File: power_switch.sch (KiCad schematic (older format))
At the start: 111 parts, among them IC1 ATTINY2313A-P, P1 CONN_2, P10 CONN_01X01, P11 CONN_02X01, P12 CONN_01X01, P13 CONN_2, P14 CONN_2, P15 CONN_2, P16 CONN_2, P17 CONN_2, P18 CONN_2, P19 CONN_2, P2 CONN_2, P20 CONN_2, P21 CONN_01X03, P3 CONN_2, P4 CONN_2, P5 CONN_2, P6 CONN_01X03, P7 CONN_01X01, P8 CONN_01X01, P9 CONN_01X01, Q1 Q_NPN_EBC, Q10 Q_NJFET_DGS, Q11 Q_NPN_EBC, Q12 Q_NPN_EBC, Q13 Q_NJFET_DGS, Q14 Q_NJFET_DGS, Q2 Q_NJFET_DGS, Q3 Q_NPN_EBC, Q4 Q_NPN_EBC, Q5 Q_NJFET_DGS, Q6 Q_NJFET_DGS, Q7 Q_NPN_EBC, Q8 Q_NPN_EBC, Q9 Q_NJFET_DGS, U1 LTV-817, U2 LTV-817, U3 LTV-817, U4 LTV-817, U5 LTV-817, U6 LM317T, U7 LTV-817, U8 LTV-817, U9 LTV-817

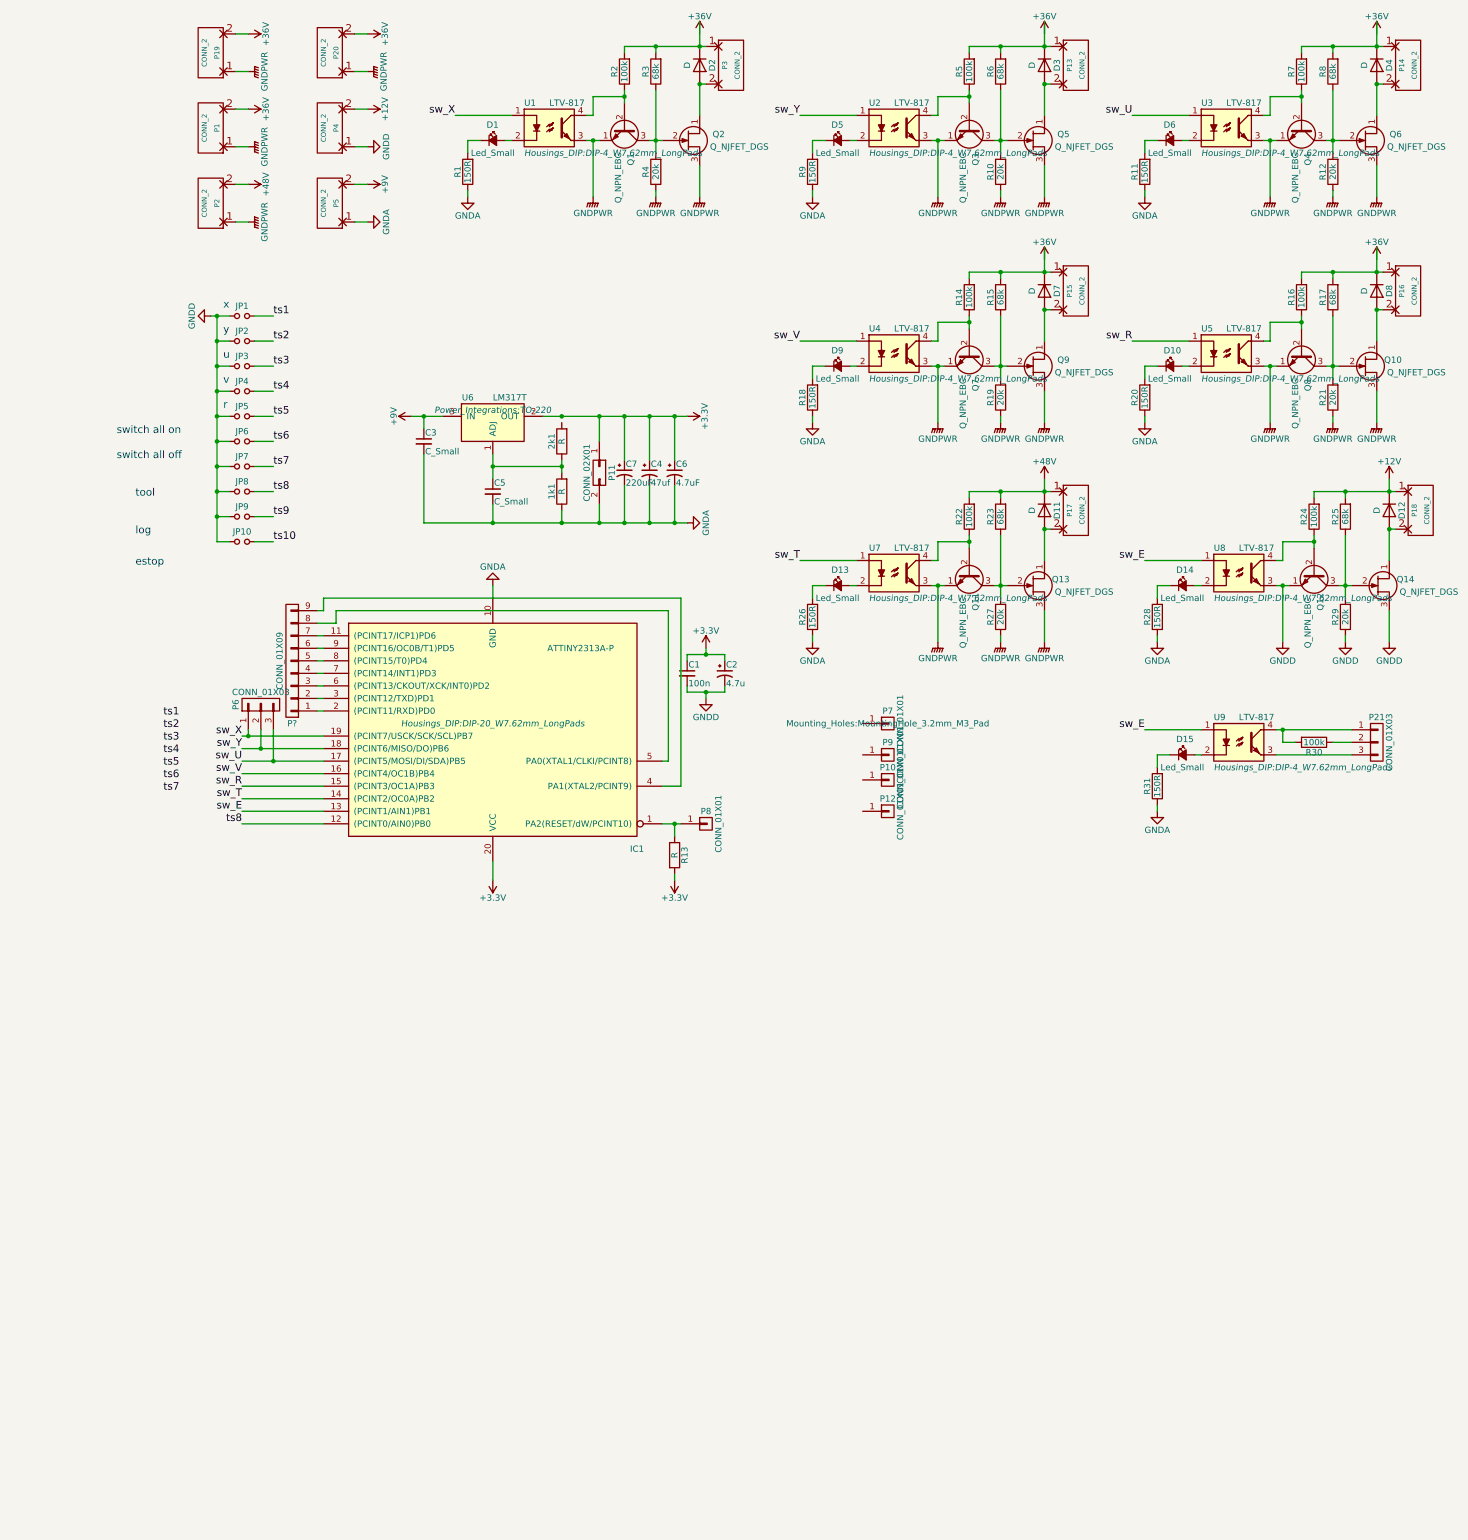
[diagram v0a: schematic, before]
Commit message: simplified version
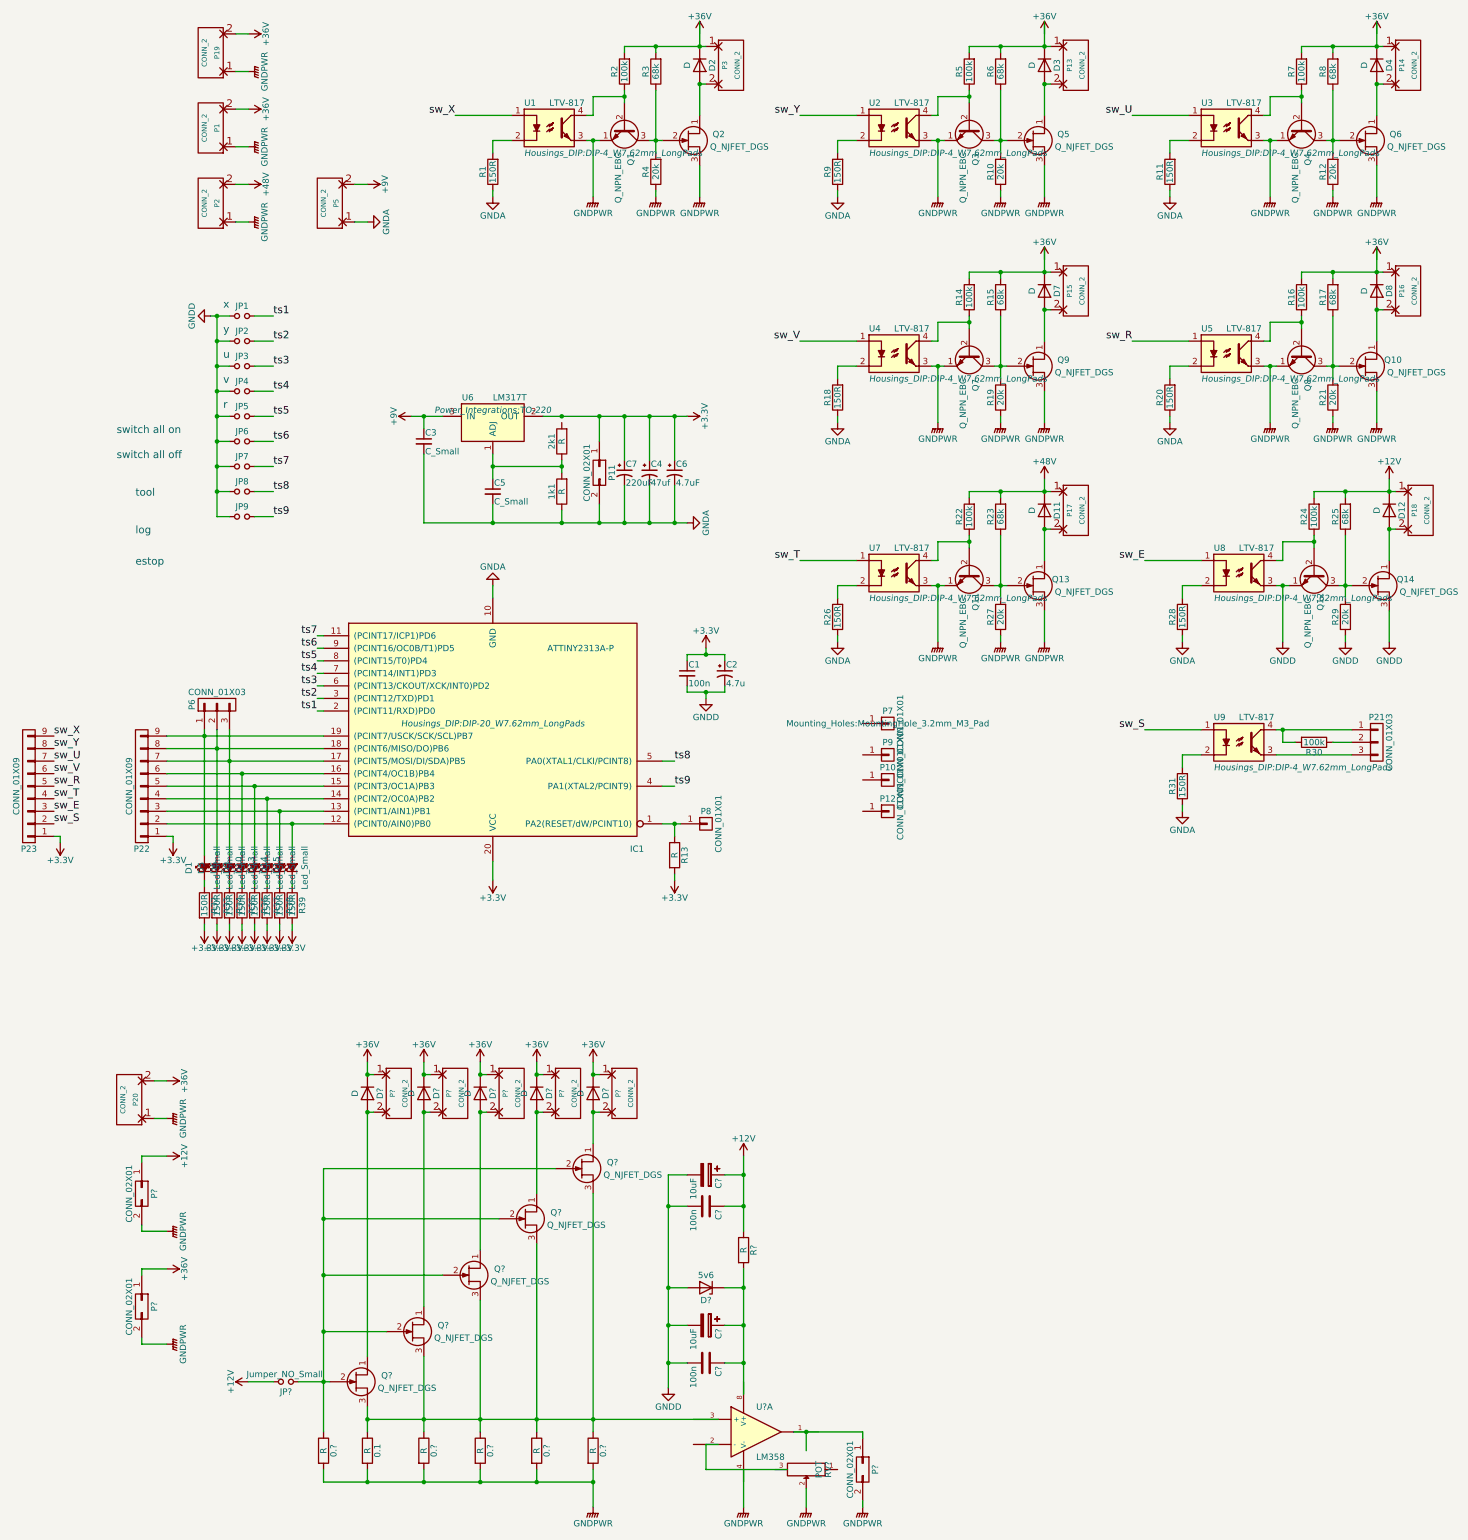
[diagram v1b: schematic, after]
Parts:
- removed JP10: Jumper_NO_Small, Buttons_Switches_ThroughHole:SW_PUSH_6mm, symbol Jumper_NO_Small
- removed P4: CONN_2, borniers:bornier2_V, symbol CONN_2-RESCUE-power_switch
- added 0.1, 0.? (x5), R?: R, symbol R
- added C? (x2): 10uF, symbol CP
- added C? (x2): 100n, symbol C
- added D?: 5v6, symbol D_Zener
- added D? (x5): D, Diodes_ThroughHole:Diode_DO-35_SOD27_Horizontal_RM10, symbol D
- added JP?: Jumper_NO_Small, symbol Jumper_NO_Small
- added P23: CONN_01X09, Socket_Strips:Socket_Strip_Straight_1x09, symbol CONN_01X09
- added P? (x5): CONN_2, borniers:bornier2_V, symbol CONN_2-RESCUE-power_switch
- added P? (x3): CONN_02X01, Pin_Headers:Pin_Header_Straight_1x02, symbol CONN_02X01
- added Q? (x5): Q_NJFET_DGS, TO_SOT_Packages_THT:TO-220_Neutral123_Vertical_LargePads, symbol Q_NJFET_DGS
- added R32, R33, R34, R35, R36, R37, R38, R39: 150R, Resistors_ThroughHole:Resistor_Horizontal_RM7mm, symbol R
- added RV?: POT, symbol POT
- added U?: LM358, symbol LM358
- P22: renamed from P?; footprint (none) -> Socket_Strips:Socket_Strip_Straight_1x09
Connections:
- net labels added: sw_S
- net labels removed: ts10
- wire segments 249 -> 324
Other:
- moved on the sheet: D1, P20, P22, P6, R1, R11, R18, R20, R26, R28, R31, R9
